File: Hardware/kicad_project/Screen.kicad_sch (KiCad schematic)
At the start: 9 parts

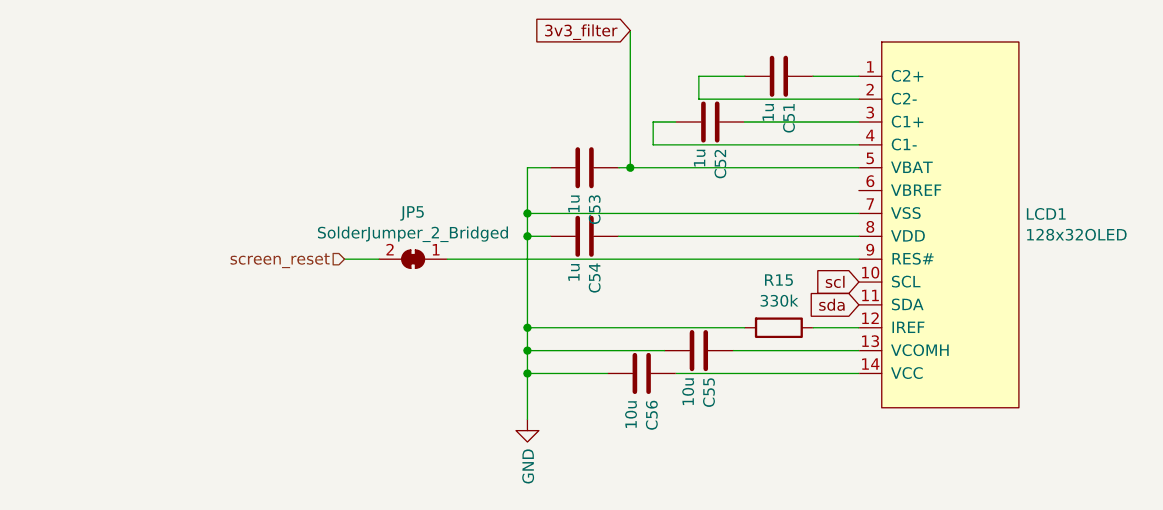
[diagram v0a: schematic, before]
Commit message: v11 hardware
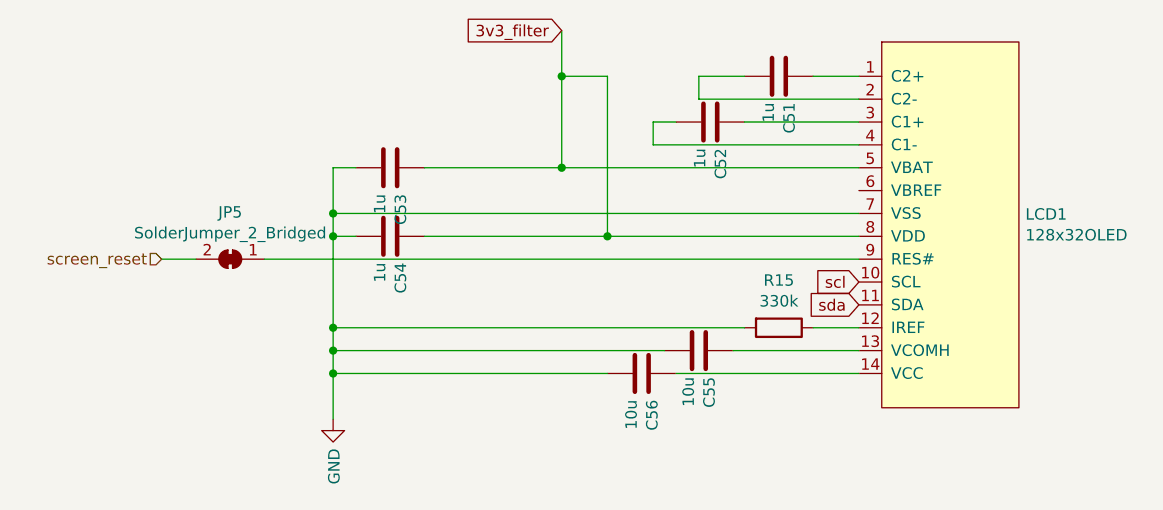
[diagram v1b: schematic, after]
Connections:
- net 3v3_filter: now also C54.1, LCD1.8 (VDD)
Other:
- moved on the sheet: C53, C54, JP5
